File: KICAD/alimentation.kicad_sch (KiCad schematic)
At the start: 17 parts, among them J2 USB_C_Receptacle_USB2.0_16P, U2 173010342, U3 CH224K

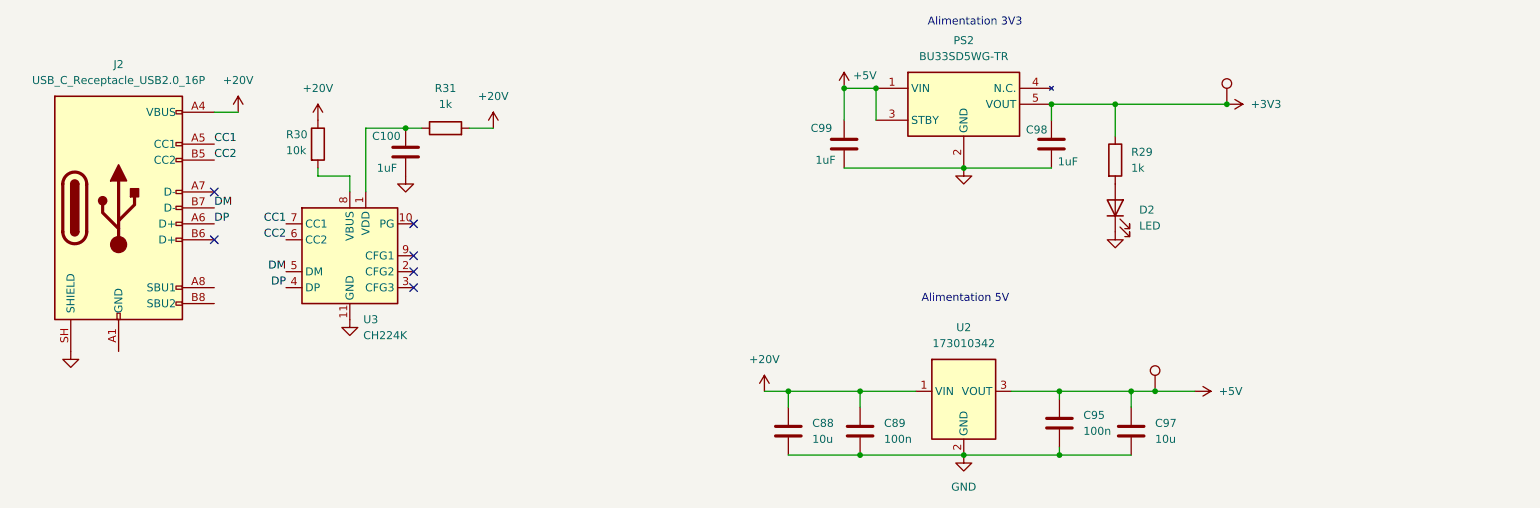
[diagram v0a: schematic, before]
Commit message: alimentatione et PLIMIT
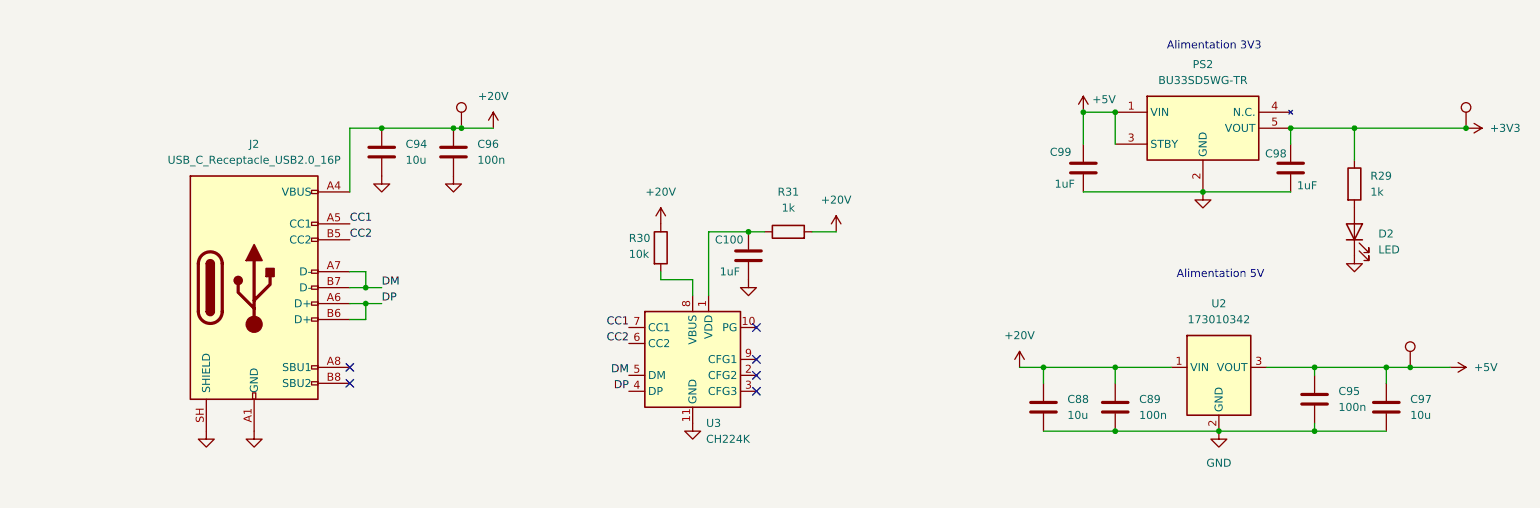
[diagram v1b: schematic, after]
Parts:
- added C94: 10u, Capacitor_SMD:C_0603_1608Metric, symbol Device:C
- added C96: 100n, Capacitor_SMD:C_0603_1608Metric, symbol Device:C
- added TP4: TestPoint, TestPoint:TestPoint_Pad_D1.5mm, symbol Connector:TestPoint
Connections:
- net +20V: now also C94.1, C96.1, TP4.1
- net DM: now also J2.A7 (D-)
- net DP: now also J2.B6 (D+)
- net GND: now also J2.A1 (GND), J2.A12 (GND), J2.B1 (GND), J2.B12 (GND), C94.2, C96.2
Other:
- moved on the sheet: C100, C88, C89, C95, C97, C98, C99, D2, J2, PS2, R29, R30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

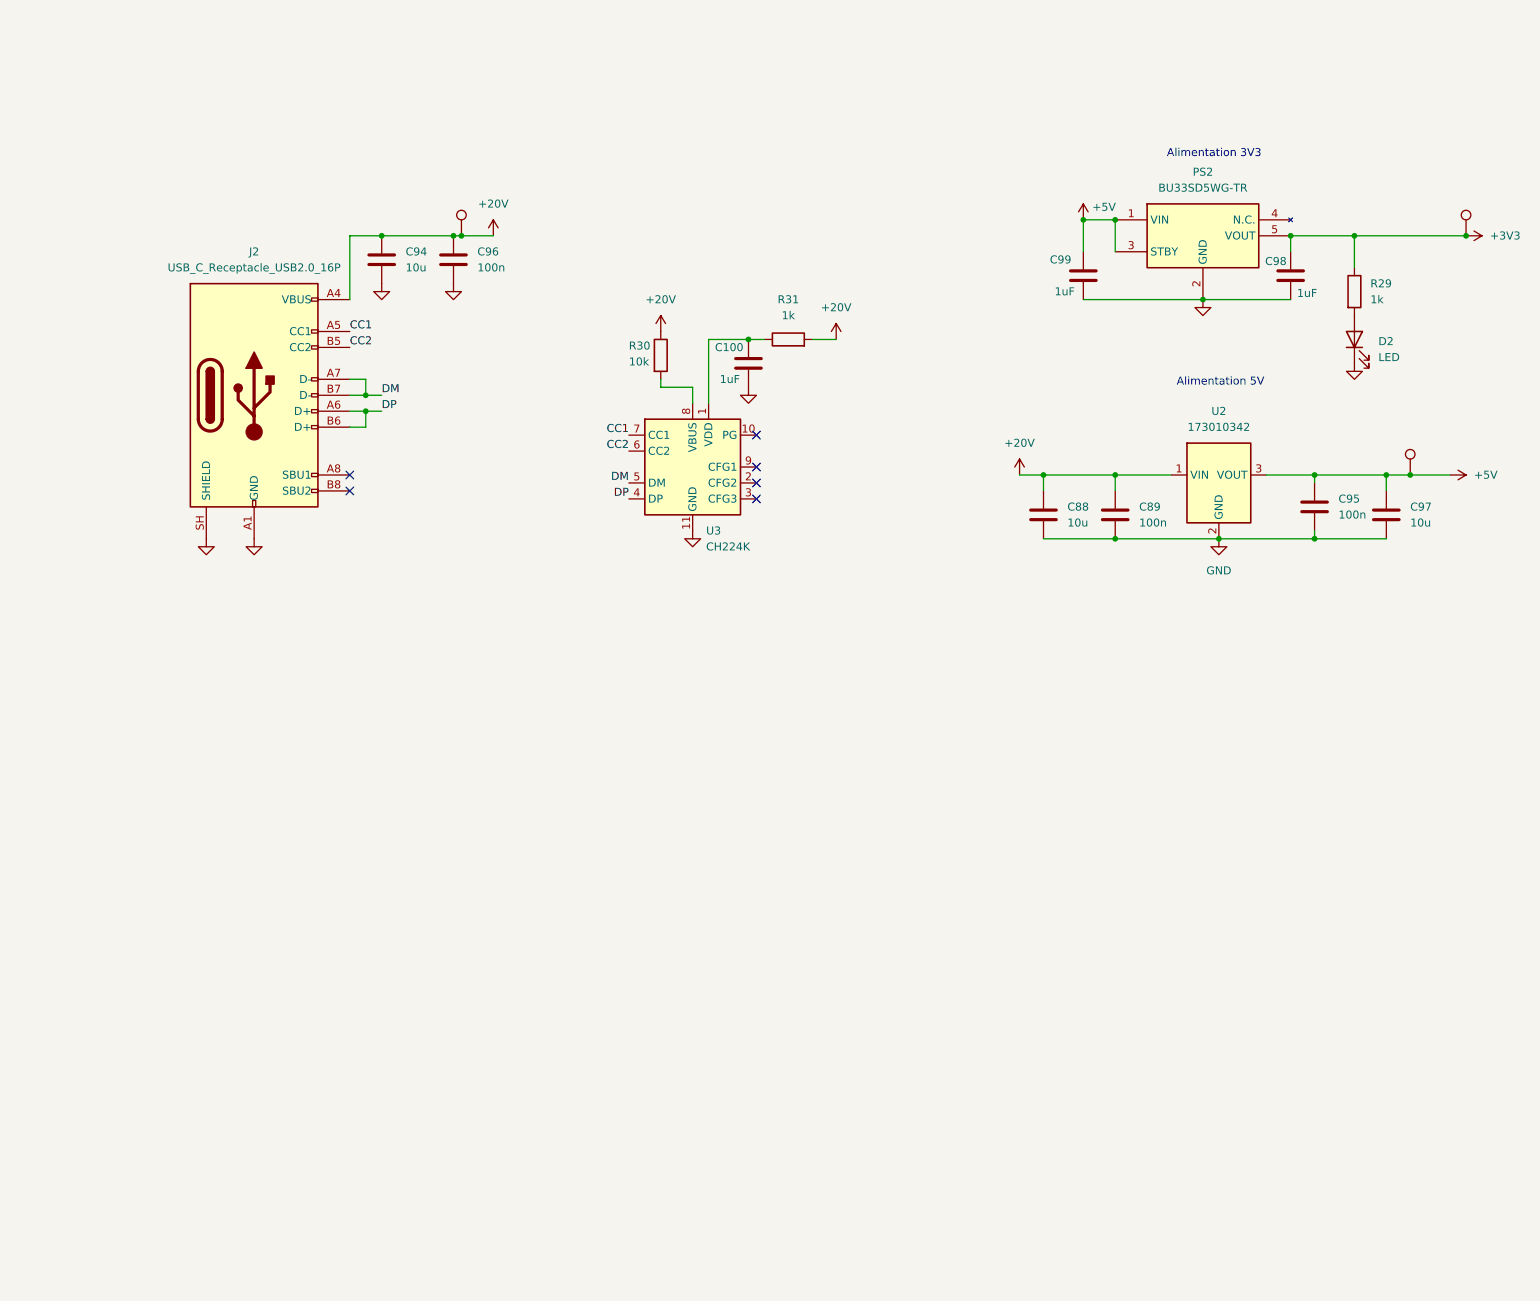
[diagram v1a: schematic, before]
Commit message: mise en forme globale
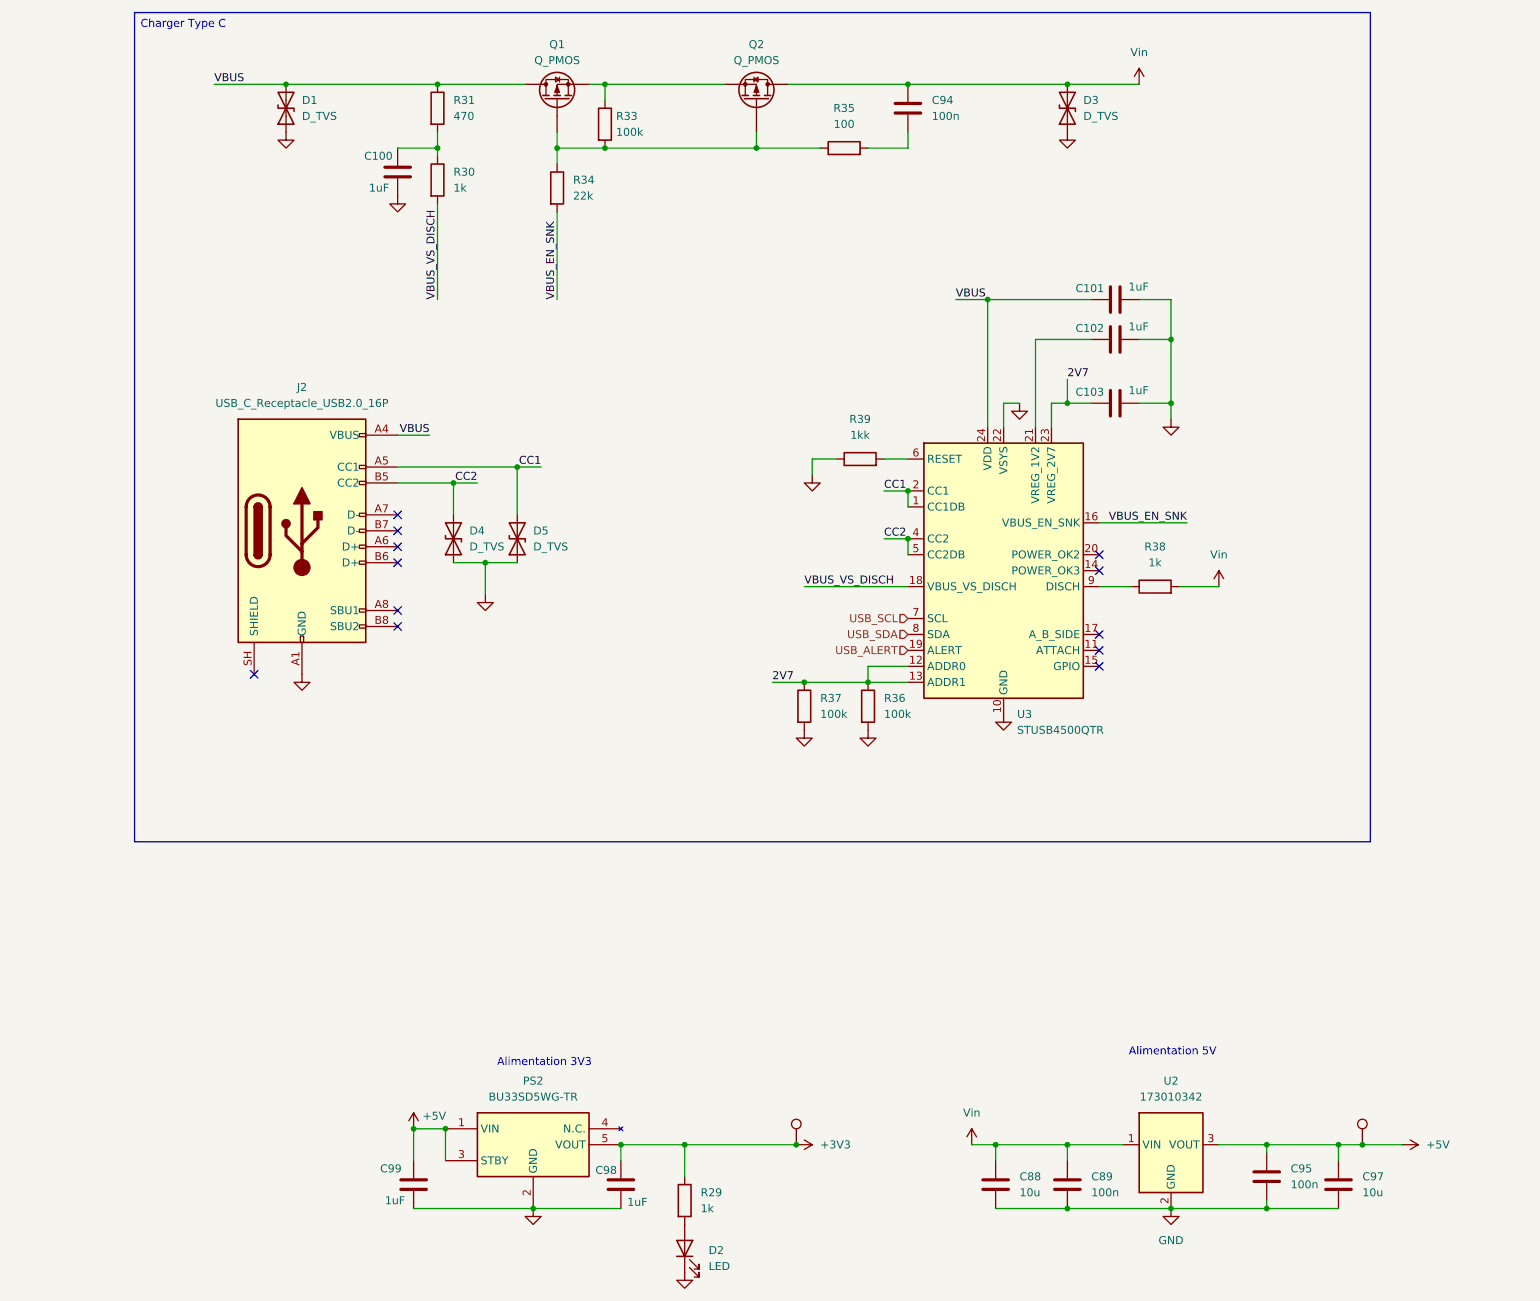
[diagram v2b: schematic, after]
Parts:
- removed C96: 100n, Capacitor_SMD:C_0603_1608Metric, symbol Device:C
- removed TP4: TestPoint, TestPoint:TestPoint_Pad_D1.5mm, symbol Connector:TestPoint
- removed U3: CH224K, Package_SO:SSOP-10-1EP_3.9x4.9mm_P1mm_EP2.1x3.3mm, symbol Interface_USB:CH224K
- added C101, C102, C103: 1uF, Capacitor_SMD:C_0603_1608Metric, symbol Device:C
- added D1, D3, D4, D5: D_TVS, symbol Device:D_TVS
- added Q1, Q2: Q_PMOS, Package_QFP:TQFP-44_10x10mm_P0.8mm, symbol Device:Q_PMOS
- added R33, R36, R37: 100k, Resistor_SMD:R_0603_1608Metric, symbol Device:R
- added R34: 22k, Resistor_SMD:R_0603_1608Metric, symbol Device:R
- added R35: 100, Resistor_SMD:R_0603_1608Metric, symbol Device:R
- added R38: 1k, Resistor_SMD:R_0603_1608Metric, symbol Device:R
- added R39: 1kk, Resistor_SMD:R_0603_1608Metric, symbol Device:R
- added U3: STUSB4500QTR, Package_DFN_QFN:QFN-24-1EP_4x4mm_P0.5mm_EP2.7x2.7mm, symbol Interface_USB:STUSB4500QTR
- C94: value 10u -> 100n
- R30: value 10k -> 1k
- R31: value 1k -> 470
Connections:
- net CC1: now also D5.2 (A2), U3.1 (CC1DB), U3.2 (CC1)
- net CC2: now also D4.2 (A2), U3.4 (CC2), U3.5 (CC2DB)
- net GND: now also C101.2, C102.2, C103.2, D1.1 (A1), D3.1 (A1), D4.1 (A1), D5.1 (A1), R36.2, R37.2, R39.1, U3.10 (GND), U3.22 (VSYS), U3.25 (GND); no longer C94.2, J2.SH (SHIELD)
- net VBUS_VS_DISCH: now reaches R30.2
- net VBUS_VS_DISCH: now also U3.18 (VBUS_VS_DISCH)
- net at C100.1: now also R30.1, R31.2; no longer R31.1
- removed net +20V: C88.1, C89.1, C94.1, J2.A4 (VBUS), J2.A9 (VBUS), J2.B4 (VBUS), J2.B9 (VBUS), R30.1, R31.2, U2.1 (VIN)
- net DM: no longer names the net of J2.A7 (D-)
- net DM: no longer J2.B7 (D-)
- net DP: no longer names the net of J2.A6 (D+)
- net DP: no longer J2.B6 (D+)
- new net: Q1.G, Q2.G, R33.2, R34.1, R35.1
- new net: C94.2, R35.2
- new net: R39.2, U3.6 (RESET)
- new net: C102.1, U3.21 (VREG_1V2)
- new net: Q1.S, Q2.S, R33.1
- new net: R38.1, U3.9 (DISCH)
- new net 2V7: C103.1, R36.1, R37.1, U3.12 (ADDR0), U3.13 (ADDR1), U3.23 (VREG_2V7)
- new net USB_ALERT: U3.19 (ALERT)
- new net USB_SCL: U3.7 (SCL)
- new net USB_SDA: U3.8 (SDA)
- new net VBUS: C101.1, D1.2 (A2), J2.A4 (VBUS), J2.A9 (VBUS), J2.B4 (VBUS), J2.B9 (VBUS), Q1.D, R31.1, U3.24 (VDD)
- new net VBUS_EN_SNK: R34.2, U3.16 (VBUS_EN_SNK)
- new net Vin: C88.1, C89.1, C94.1, D3.2 (A2), Q2.D, R38.2, U2.1 (VIN)
- no-connect marks 6 -> 12
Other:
- moved on the sheet: C88, C89, C95, C97, C98, C99, D2, J2, PS2, R29, U2
